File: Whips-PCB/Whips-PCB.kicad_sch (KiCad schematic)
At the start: 29 parts, among them J1 12 VDC, J2 RS422 BUS, J3 SPEAKER 4OHM, J4 TO WHIP, J5 RS422 BUS, SW2 SW_DIP_x06, U2 MAX485ESA+T, U3 SN74AHCT125DR, U4 TSR_1-2450, U5 MAX98357AETE+T, U6 Teensy4.1_Minimal

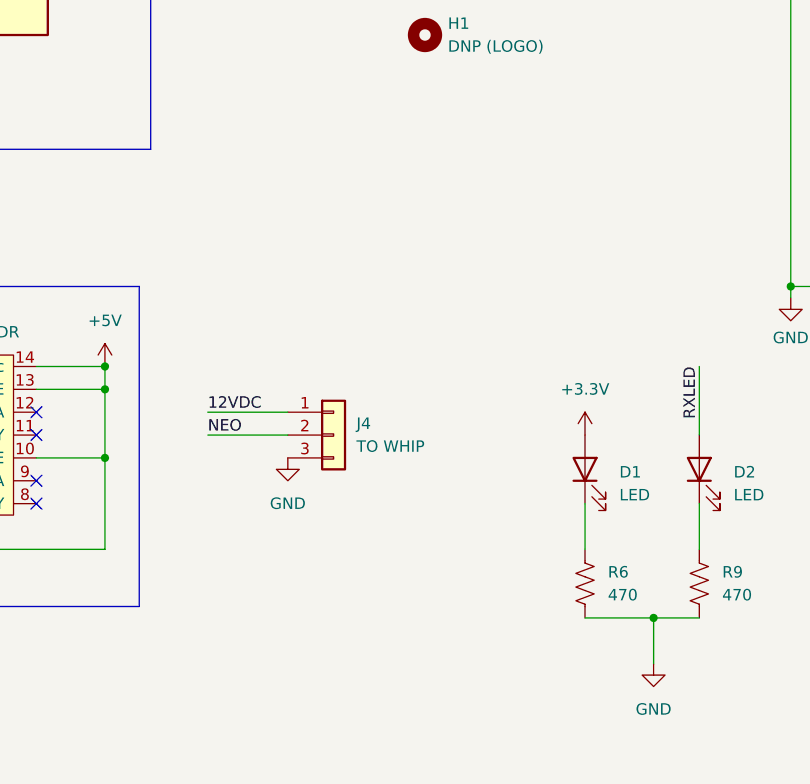
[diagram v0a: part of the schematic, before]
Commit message: Much better turtle logo with backlights
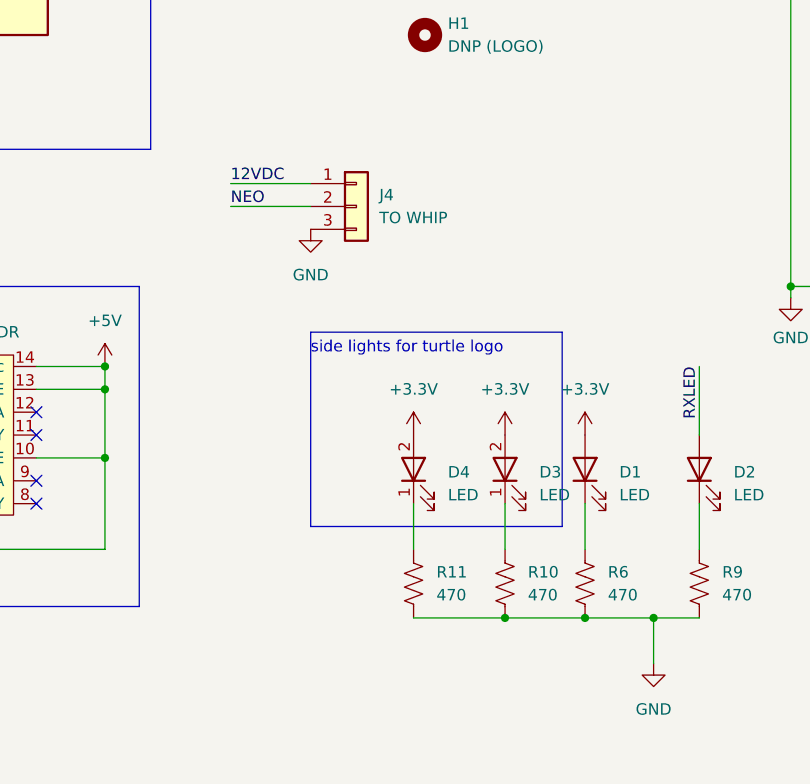
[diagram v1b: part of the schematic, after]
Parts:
- added D3, D4: LED, Joels KiCad Footprint Library:Everlight 99-218GLM2C-L7277SGU-TR8-T0-ES side view LED, symbol Device:LED
- added R10, R11: 470, Resistor_SMD:R_0402_1005Metric, symbol Device:R_US
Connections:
- net +3.3V: now also D3.2 (A), D4.2 (A)
- net GND: now also R10.2, R11.2
- new net: D3.1 (K), R10.1
- new net: D4.1 (K), R11.1
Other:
- note added: "side lights for turtle logo"
- moved on the sheet: J4
